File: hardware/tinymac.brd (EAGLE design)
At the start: 43 x 41.4 mm, 29 parts, among them IC1 LPC1114FN28, J1 ZX62-B-5PA, SW1 TACT_SW, SW2 TACT_SW, SW3 TACT_SW, SW4 TACT_SW, SW5 TACT_SW, T1 TA48M033F

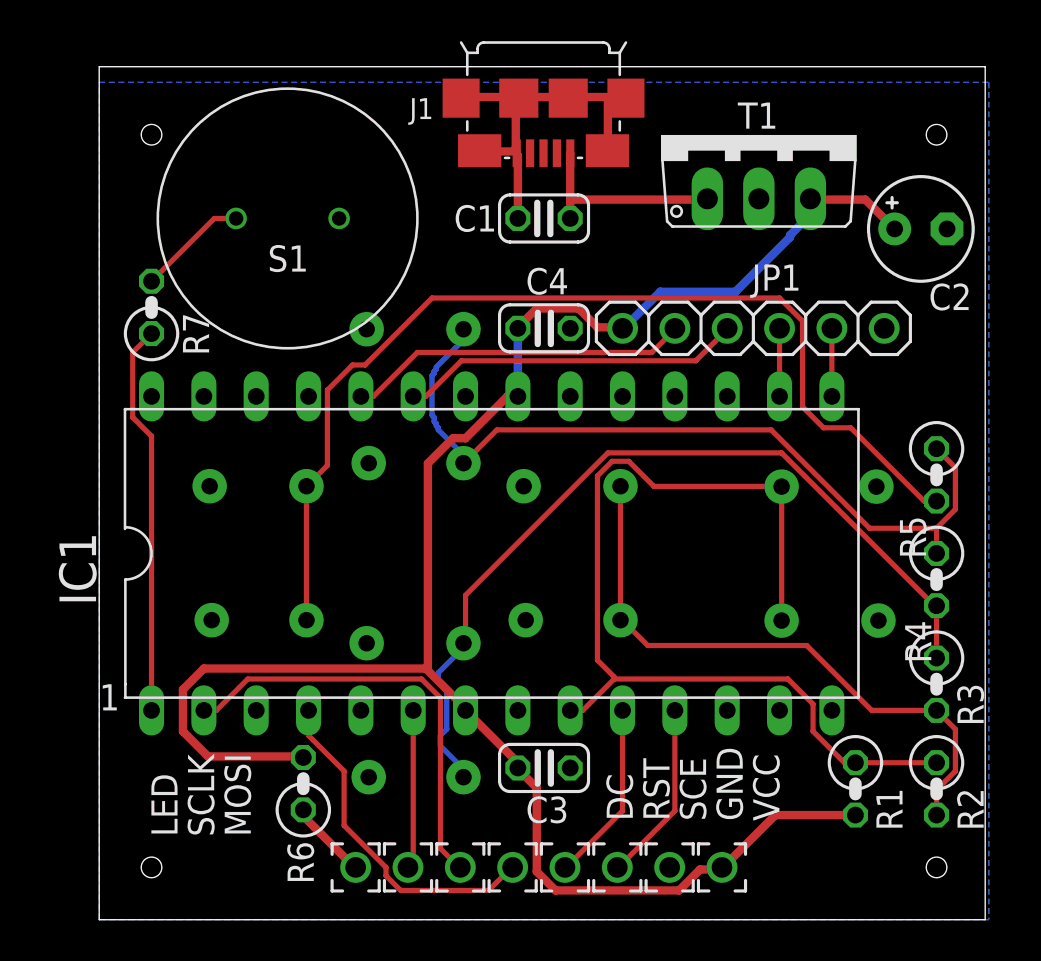
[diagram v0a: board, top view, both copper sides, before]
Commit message: change eagleup output setting
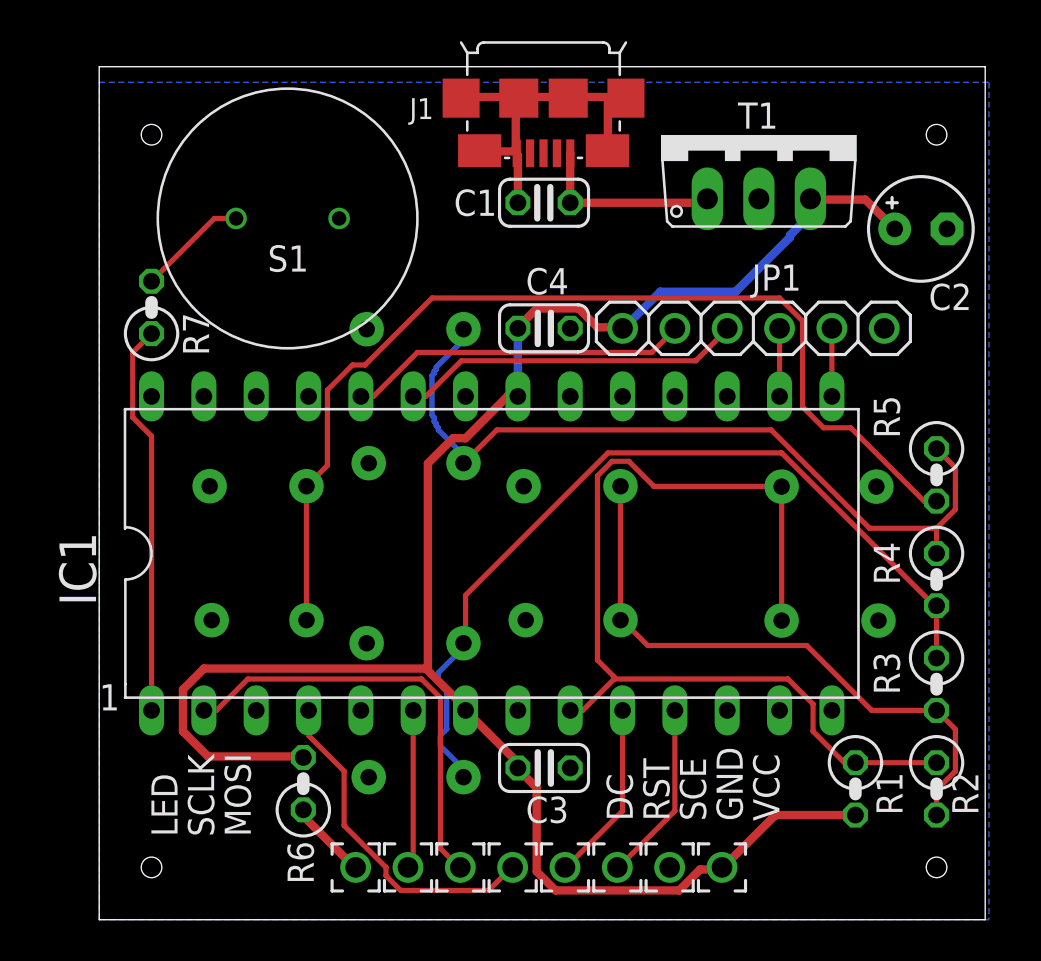
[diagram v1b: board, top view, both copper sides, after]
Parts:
- moved C1 0.76 mm to (21.6, 34.8)
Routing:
- net GND: track 19.3 -> 18.6 mm
- net VBUS: track 9.83 -> 9.31 mm
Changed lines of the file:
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@@
 <setting verticaltext="up"/>
 </settings>
-<grid distance="0.1" unitdist="inch" unit="inch" style="lines" multiple="1" display="yes" altdistance="0.01" altunitdist="inch" altunit="inch"/>
+<grid distance="0.1" unitdist="inch" unit="mm" style="lines" multiple="1" display="yes" altdistance="0.01" altunitdist="inch" altunit="inch"/>
 <layers>
 <layer number="1" name="Top" color="4" fill="1" visible="yes" active="yes"/>
@@
 <attribute name="NAME" x="31" y="38.3928" size="1.27" layer="25" ratio="10"/>
 </element>
-<element name="C1" library="tinymac" package="C025-024X044" value="0.1uF" x="21.59" y="34.036" smashed="yes" rot="R180">
-<attribute name="NAME" x="19.304" y="34.671" size="1.27" layer="25" ratio="10" rot="R180"/>
+<element name="C1" library="tinymac" package="C025-024X044" value="0.1uF" x="21.59" y="34.798" smashed="yes" rot="R180">
+<attribute name="NAME" x="19.304" y="35.433" size="1.27" layer="25" ratio="10" rot="R180"/>
 </element>
 <element name="C2" library="tinymac" package="E2,5-5" value="47uF" x="39.878" y="33.528" smashed="yes">
@@
 <attribute name="NAME" x="9.282" y="11.794" size="1.27" layer="26" rot="MR0"/>
 </element>
-<element name="R1" library="tinymac" package="0207/2V" value="10K" x="36.703" y="6.35" rot="R270"/>
-<element name="R2" library="tinymac" package="0207/2V" value="2.4K" x="40.64" y="6.35" rot="R270"/>
-<element name="R3" library="tinymac" package="0207/2V" value="4.3K" x="40.64" y="11.43" rot="R270"/>
+<element name="R1" library="tinymac" package="0207/2V" value="10K" x="36.703" y="6.35" smashed="yes" rot="R270">
+<attribute name="NAME" x="37.719" y="7.1628" size="1.27" layer="25" ratio="10" rot="R270"/>
+</element>
+<element name="R2" library="tinymac" package="0207/2V" value="2.4K" x="40.64" y="6.35" smashed="yes" rot="R270">
+<attribute name="NAME" x="41.402" y="7.1628" size="1.27" layer="25" ratio="10" rot="R270"/>
+</element>
+<element name="R3" library="tinymac" package="0207/2V" value="4.3K" x="40.64" y="11.43" smashed="yes" rot="R270">
+<attribute name="NAME" x="37.592" y="13.0048" size="1.27" layer="25" ratio="10" rot="R270"/>
+</element>
 <element name="R4" library="tinymac" package="0207/2V" value="8.2K" x="40.64" y="16.51" smashed="yes" rot="R270">
-<attribute name="NAME" x="39.116" y="14.5288" size="1.27" layer="25" ratio="10" rot="R270"/>
+<attribute name="NAME" x="37.592" y="18.3388" size="1.27" layer="25" ratio="10" rot="R270"/>
 </element>
 <element name="R5" library="tinymac" package="0207/2V" value="24K" x="40.64" y="21.59" smashed="yes" rot="R270">
-<attribute name="NAME" x="38.862" y="19.6088" size="1.27" layer="25" ratio="10" rot="R270"/>
+<attribute name="NAME" x="37.592" y="25.4508" size="1.27" layer="25" ratio="10" rot="R270"/>
 </element>
 <element name="C4" library="tinymac" package="C025-024X044" value="0.1uF" x="21.59" y="28.702" smashed="yes">
@@
 <wire x1="20.2184" y1="37.4904" x2="20.264" y2="37.2" width="0.4064" layer="1"/>
 <wire x1="20.2184" y1="39.7256" x2="20.364" y2="39.875" width="0.4064" layer="1"/>
-<wire x1="20.32" y1="34.036" x2="20.32" y2="37.084" width="0.4064" layer="1"/>
 <wire x1="20.32" y1="37.084" x2="20.264" y2="37.2" width="0.4064" layer="1"/>
+<wire x1="20.32" y1="37.084" x2="20.32" y2="34.798" width="0.4064" layer="1"/>
 </signal>
 <signal name="N$15">
@@
 <contactref element="T1" pad="1"/>
 <contactref element="C1" pad="1"/>
-<wire x1="22.86" y1="34.036" x2="22.86" y2="34.9504" width="0.4064" layer="1"/>
-<wire x1="22.86" y1="34.9504" x2="22.86" y2="37.1856" width="0.4064" layer="1"/>
 <wire x1="22.86" y1="37.1856" x2="22.864" y2="37.2" width="0.4064" layer="1"/>
-<wire x1="22.86" y1="34.9504" x2="29.464" y2="34.9504" width="0.4064" layer="1"/>
 <wire x1="29.464" y1="34.9504" x2="29.516" y2="34.988" width="0.4064" layer="1"/>
+<wire x1="22.86" y1="37.1856" x2="22.86" y2="34.798" width="0.4064" layer="1"/>
+<wire x1="22.86" y1="34.798" x2="29.516" y2="34.798" width="0.4064" layer="1"/>
+<wire x1="29.516" y1="34.798" x2="29.516" y2="34.988" width="0.4064" layer="1"/>
 </signal>
 <signal name="N$2">

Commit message: change DRU setting to Seeed-2layer-DRU
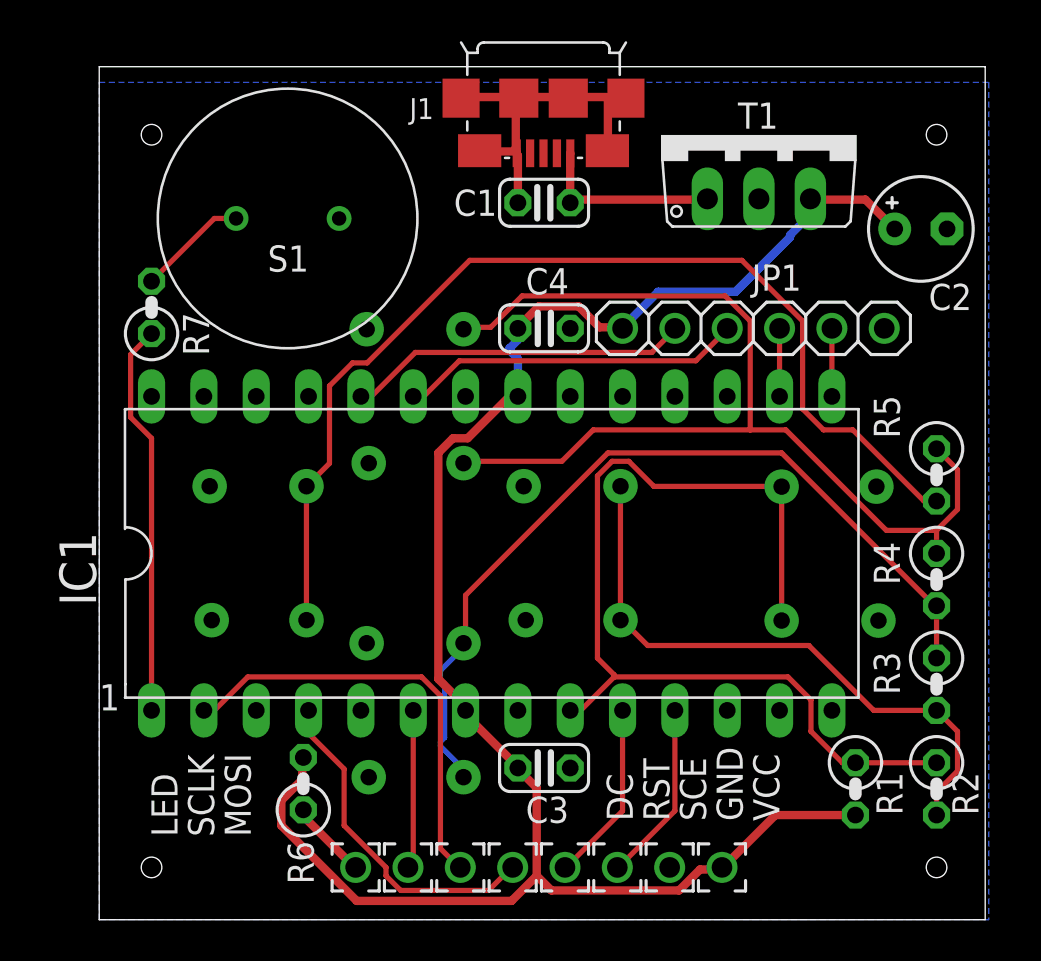
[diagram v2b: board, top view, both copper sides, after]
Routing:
- net N$7: track 39.2 -> 51.9 mm
- net +3.3V: track 92.0 -> 89.6 mm
- net N$8: track 49.5 -> 51.2 mm
